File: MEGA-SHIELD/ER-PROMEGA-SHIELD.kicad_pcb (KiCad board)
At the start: 2 copper layers, 80 parts, among them J1 12V, J10 Screw_Terminal_01x10, J11 Screw_Terminal_01x07, J12 Conn_01x03_Female, J13 Screw_Terminal_01x04, J14 Conn_01x03_Female, J15 Screw_Terminal_01x04, J16 Conn_01x03_Female, J17 Screw_Terminal_01x04, J18 1x3, J19 Screw_Terminal_01x07, J2 Conn_01x03_Female, J3 Screw_Terminal_01x04, J4 Screw_Terminal_01x10, J5 Screw_Terminal_01x06, J6 Screw_Terminal_01x06, J7 Screw_Terminal_01x10, J8 Screw_Terminal_01x04, J9 Screw_Terminal_01x10, K1 G5LE-1, K2 G5LE-1, K3 G5LE-1, K4 G5LE-1, Q1 2N7002H, Q2 2N7002H, Q3 2N7002H, Q4 2N7002H, U1 PC817, U2 PC817, U3 PC817, U4 PC817

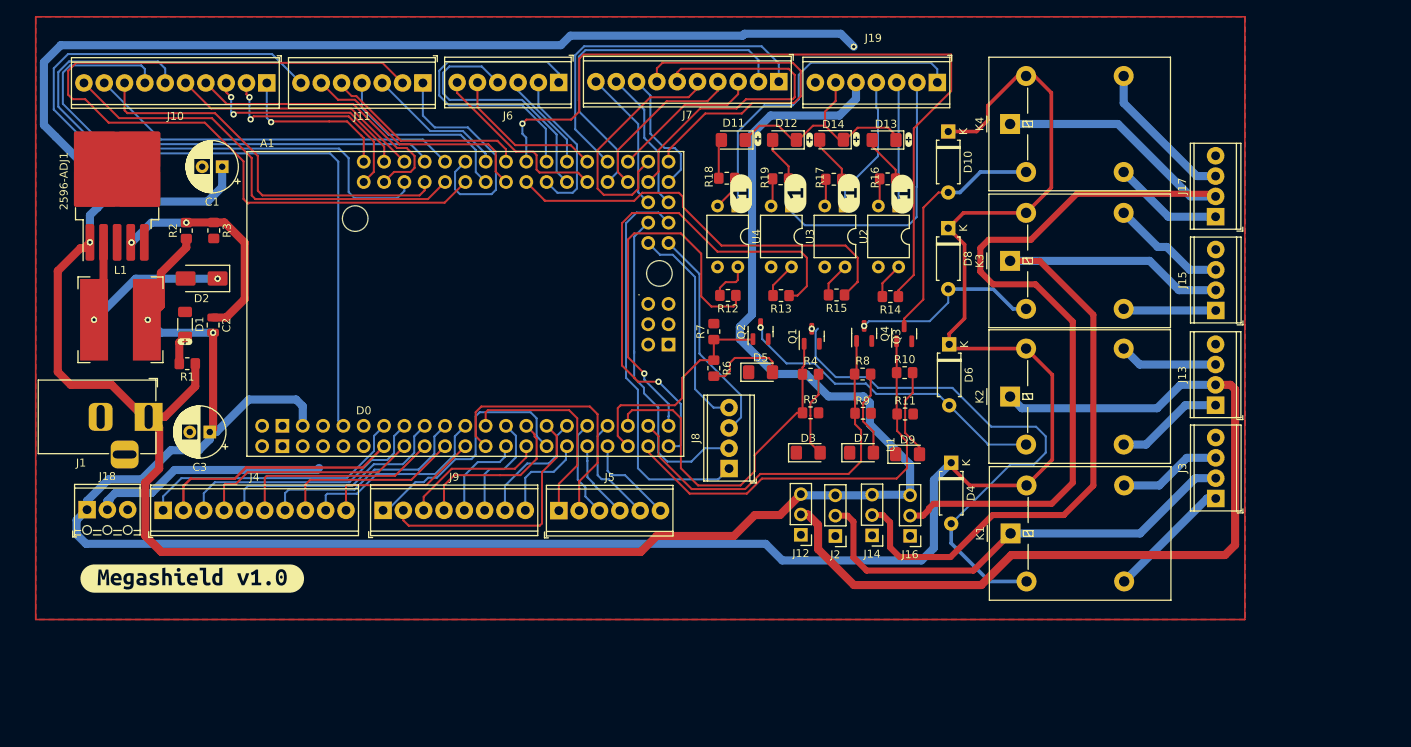
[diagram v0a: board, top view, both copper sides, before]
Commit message: develop: version 1.1
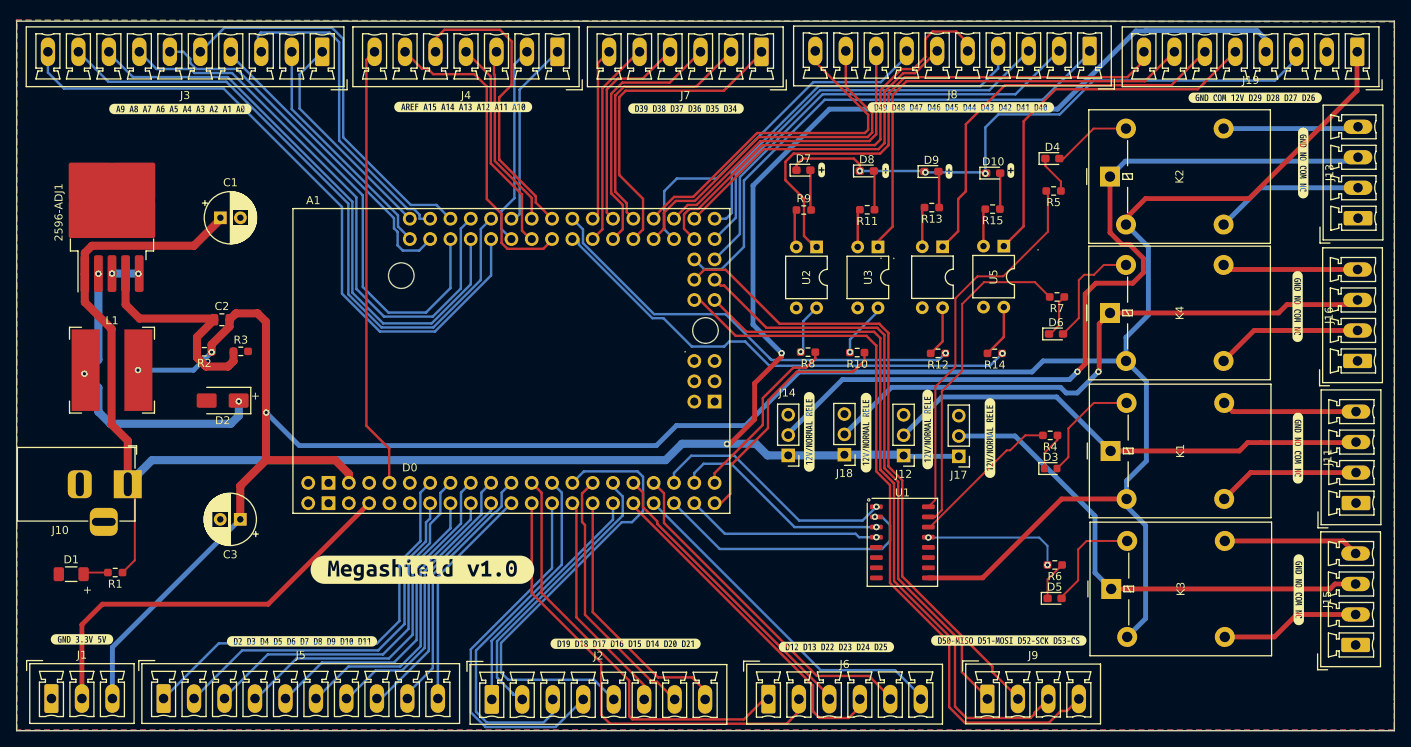
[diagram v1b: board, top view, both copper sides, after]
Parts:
- removed the D10 at (186.6, 73.1)
- removed the D7 at (175.7, 113.3)
- removed the D8 at (186.6, 85.2)
- removed the D9 at (181.5, 113.5)
- removed the J2 at (172.5, 123.7)
- removed the J3 at (220.0, 119.0)
- removed Q1, Q2, Q3, Q4: 2N7002H, Package_TO_SOT_SMD:SOT-23
- removed the R10 at (181.1, 103.3)
- removed the R11 at (181.2, 108.4)
- removed the R8 at (175.9, 103.4)
- removed the R9 at (175.9, 108.3)
- removed kibuzzard-653EC514 (x4): G***, kibuzzard-653EC514
- removed the kibuzzard-653EC60C at (91.2, 99.4)
- added J11: Screw_Terminal_01x03, Connector_Phoenix_MC:PhoenixContact_MCV_1,5_4-G-3.81_1x04_P3.81mm_Vertical, F.Cu at (237.6, 119.6)
- added J18: Conn_01x03_Female, Connector_PinHeader_2.54mm:PinHeader_1x03_P2.54mm_Vertical, F.Cu at (173.6, 113.5)
- added U1: ULN2003, PCM_Package_SO_AKL:SOP-16_4.55x10.3mm_P1.27mm, F.Cu at (180.8, 124.5)
- added kibuzzard-65BC3466: G***, kibuzzard-65BC3466, F.Cu at (90.6, 70.3)
- added kibuzzard-65BC3498: G***, kibuzzard-65BC3498, F.Cu at (126.0, 70.0)
- added kibuzzard-65BC34CA: G***, kibuzzard-65BC34CA, F.Cu at (153.8, 70.2)
- added kibuzzard-65BC34FE: G***, kibuzzard-65BC34FE, F.Cu at (188.2, 70.1)
- added kibuzzard-65BC3573: G***, kibuzzard-65BC3573, F.Cu at (224.9, 68.9)
- added kibuzzard-65BC35D6: G***, kibuzzard-65BC35D6, F.Cu at (78.3, 136.6)
- added kibuzzard-65BC363F: G***, kibuzzard-65BC363F, F.Cu at (105.8, 136.8)
- added kibuzzard-65BC3690: G***, kibuzzard-65BC3690, F.Cu at (146.2, 137.2)
- added kibuzzard-65BC36E0: G***, kibuzzard-65BC36E0, F.Cu at (172.6, 137.6)
- added kibuzzard-65BC3745: G***, kibuzzard-65BC3745, F.Cu at (194.2, 136.8)
- added kibuzzard-65BC37BD: G***, kibuzzard-65BC37BD, F.Cu at (176.3, 110.8)
- added kibuzzard-65BC37BD: G***, kibuzzard-65BC37BD, F.Cu at (169.2, 110.7)
- added kibuzzard-65BC37BD: G***, kibuzzard-65BC37BD, F.Cu at (184.0, 110.4)
- added kibuzzard-65BC37BD: G***, kibuzzard-65BC37BD, F.Cu at (191.8, 111.4)
- added kibuzzard-65BC3814: G***, kibuzzard-65BC3814, F.Cu at (230.4, 130.4)
- added kibuzzard-65BC3814: G***, kibuzzard-65BC3814, F.Cu at (230.9, 77.0)
- added kibuzzard-65BC3814: G***, kibuzzard-65BC3814, F.Cu at (230.2, 95.0)
- added kibuzzard-65BC3814: G***, kibuzzard-65BC3814, F.Cu at (230.3, 112.7)
- 2596-ADJ1: value LM2596S-5 -> REGULADOR ADJ
- D10: renamed from D14; footprint LED_SMD:LED_1206_3216Metric_Pad1.42x1.75mm_HandSolder -> LED_SMD:LED_0603_1608Metric_Pad1.05x0.95mm_HandSolder
- D3: value LEDRELE -> LED; footprint LED_SMD:LED_1206_3216Metric_Pad1.42x1.75mm_HandSolder -> LED_SMD:LED_0603_1608Metric
- D4, D6: value 1N5400 -> LED; footprint Diode_THT:D_A-405_P7.62mm_Horizontal -> LED_SMD:LED_0603_1608Metric_Pad1.05x0.95mm_HandSolder
- D5: value LEDRELE -> LED; footprint LED_SMD:LED_1206_3216Metric_Pad1.42x1.75mm_HandSolder -> LED_SMD:LED_0603_1608Metric_Pad1.05x0.95mm_HandSolder
- D7: renamed from D11; footprint LED_SMD:LED_1206_3216Metric_Pad1.42x1.75mm_HandSolder -> LED_SMD:LED_0603_1608Metric_Pad1.05x0.95mm_HandSolder
- D8: renamed from D12; footprint LED_SMD:LED_1206_3216Metric_Pad1.42x1.75mm_HandSolder -> LED_SMD:LED_0603_1608Metric_Pad1.05x0.95mm_HandSolder
- D9: renamed from D13; footprint LED_SMD:LED_1206_3216Metric_Pad1.42x1.75mm_HandSolder -> LED_SMD:LED_0603_1608Metric_Pad1.05x0.95mm_HandSolder
- J1: renamed from J18; footprint TerminalBlock_Phoenix:TerminalBlock_Phoenix_MPT-0,5-3-2.54_1x03_P2.54mm_Horizontal -> Connector_Phoenix_MC:PhoenixContact_MCV_1,5_3-G-3.81_1x03_P3.81mm_Vertical
- J13, J15: value Screw_Terminal_01x04 -> Screw_Terminal_01x03; footprint TerminalBlock_Phoenix:TerminalBlock_Phoenix_MPT-0,5-4-2.54_1x04_P2.54mm_Horizontal -> Connector_Phoenix_MC:PhoenixContact_MCV_1,5_4-G-3.81_1x04_P3.81mm_Vertical
- J16: value Conn_01x03_Female -> Screw_Terminal_01x03; footprint Connector_PinHeader_2.54mm:PinHeader_1x03_P2.54mm_Vertical -> Connector_Phoenix_MC:PhoenixContact_MCV_1,5_4-G-3.81_1x04_P3.81mm_Vertical
- J17: value Screw_Terminal_01x04 -> Conn_01x03_Female; footprint TerminalBlock_Phoenix:TerminalBlock_Phoenix_MPT-0,5-4-2.54_1x04_P2.54mm_Horizontal -> Connector_PinHeader_2.54mm:PinHeader_1x03_P2.54mm_Vertical
- J19: value Screw_Terminal_01x07 -> ENTRADAS OPTOS; footprint TerminalBlock_Phoenix:TerminalBlock_Phoenix_MPT-0,5-7-2.54_1x07_P2.54mm_Horizontal -> Connector_Phoenix_MC:PhoenixContact_MCV_1,5_8-G-3.81_1x08_P3.81mm_Vertical
- J2: renamed from J9; footprint TerminalBlock_Phoenix:TerminalBlock_Phoenix_MPT-0,5-8-2.54_1x08_P2.54mm_Horizontal -> Connector_Phoenix_MC:PhoenixContact_MCV_1,5_8-G-3.81_1x08_P3.81mm_Vertical
- J3: renamed from J10; footprint TerminalBlock_Phoenix:TerminalBlock_Phoenix_MPT-0,5-10-2.54_1x10_P2.54mm_Horizontal -> Connector_Phoenix_MC:PhoenixContact_MCV_1,5_10-G-3.81_1x10_P3.81mm_Vertical
- J4: renamed from J11; footprint TerminalBlock_Phoenix:TerminalBlock_Phoenix_MPT-0,5-7-2.54_1x07_P2.54mm_Horizontal -> Connector_Phoenix_MC:PhoenixContact_MCV_1,5_7-G-3.81_1x07_P3.81mm_Vertical
- J5: renamed from J4; footprint TerminalBlock_Phoenix:TerminalBlock_Phoenix_MPT-0,5-10-2.54_1x10_P2.54mm_Horizontal -> Connector_Phoenix_MC:PhoenixContact_MCV_1,5_10-G-3.81_1x10_P3.81mm_Vertical
- J6: renamed from J5; footprint TerminalBlock_Phoenix:TerminalBlock_Phoenix_MPT-0,5-6-2.54_1x06_P2.54mm_Horizontal -> Connector_Phoenix_MC:PhoenixContact_MCV_1,5_6-G-3.81_1x06_P3.81mm_Vertical
- J7: renamed from J6; footprint TerminalBlock_Phoenix:TerminalBlock_Phoenix_MPT-0,5-6-2.54_1x06_P2.54mm_Horizontal -> Connector_Phoenix_MC:PhoenixContact_MCV_1,5_6-G-3.81_1x06_P3.81mm_Vertical
- J8: renamed from J7; footprint TerminalBlock_Phoenix:TerminalBlock_Phoenix_MPT-0,5-10-2.54_1x10_P2.54mm_Horizontal -> Connector_Phoenix_MC:PhoenixContact_MCV_1,5_10-G-3.81_1x10_P3.81mm_Vertical
- J9: renamed from J8; footprint TerminalBlock_Phoenix:TerminalBlock_Phoenix_MPT-0,5-4-2.54_1x04_P2.54mm_Horizontal -> Connector_Phoenix_MC:PhoenixContact_MCV_1,5_4-G-3.81_1x04_P3.81mm_Vertical
- K1: value G5LE-1 -> Rele3
- K2: value G5LE-1 -> Rele1
- K3: value G5LE-1 -> Rele4
- K4: value G5LE-1 -> Rele2
- R1, R2, R3: footprint Resistor_SMD:R_0805_2012Metric_Pad1.20x1.40mm_HandSolder -> Resistor_SMD:R_0603_1608Metric_Pad0.98x0.95mm_HandSolder
- R10: renamed from R13; footprint Resistor_SMD:R_0805_2012Metric_Pad1.20x1.40mm_HandSolder -> Resistor_SMD:R_0603_1608Metric_Pad0.98x0.95mm_HandSolder
- R11: renamed from R19; footprint Resistor_SMD:R_0805_2012Metric_Pad1.20x1.40mm_HandSolder -> Resistor_SMD:R_0603_1608Metric_Pad0.98x0.95mm_HandSolder
- R12: renamed from R14; footprint Resistor_SMD:R_0805_2012Metric_Pad1.20x1.40mm_HandSolder -> Resistor_SMD:R_0603_1608Metric_Pad0.98x0.95mm_HandSolder
- R13: renamed from R16; footprint Resistor_SMD:R_0805_2012Metric_Pad1.20x1.40mm_HandSolder -> Resistor_SMD:R_0603_1608Metric_Pad0.98x0.95mm_HandSolder
- R14: renamed from R15; footprint Resistor_SMD:R_0805_2012Metric_Pad1.20x1.40mm_HandSolder -> Resistor_SMD:R_0603_1608Metric_Pad0.98x0.95mm_HandSolder
- R15: renamed from R17; footprint Resistor_SMD:R_0805_2012Metric_Pad1.20x1.40mm_HandSolder -> Resistor_SMD:R_0603_1608Metric_Pad0.98x0.95mm_HandSolder
- R4, R6: value 1k -> R; footprint Resistor_SMD:R_0805_2012Metric_Pad1.20x1.40mm_HandSolder -> Resistor_SMD:R_0603_1608Metric_Pad0.98x0.95mm_HandSolder
- R5, R7: value 10K -> R; footprint Resistor_SMD:R_0805_2012Metric_Pad1.20x1.40mm_HandSolder -> Resistor_SMD:R_0603_1608Metric_Pad0.98x0.95mm_HandSolder
- R8: renamed from R12; footprint Resistor_SMD:R_0805_2012Metric_Pad1.20x1.40mm_HandSolder -> Resistor_SMD:R_0603_1608Metric_Pad0.98x0.95mm_HandSolder
- R9: renamed from R18; footprint Resistor_SMD:R_0805_2012Metric_Pad1.20x1.40mm_HandSolder -> Resistor_SMD:R_0603_1608Metric_Pad0.98x0.95mm_HandSolder
- U2: renamed from U4; value PC817 -> OPTO1
- U3: value PC817 -> OPTO2
- U4: renamed from U1; value PC817 -> OPTO3
- U5: renamed from U2; value PC817 -> OPTO4
- moved J16 60.1 mm to (237.7, 101.8), turned to 90 degrees
- moved J19 52.6 mm to (237.7, 63.1)
- moved R6 49.2 mm to (199.9, 127.3), turned to 180 degrees
- moved D5 46.4 mm to (199.9, 131.5)
- moved J15 45.3 mm to (237.5, 137.3)
- moved J17 43.9 mm to (187.9, 113.7), turned to 180 degrees
- moved J9 43.3 mm to (191.5, 144.1), turned to 0 degrees
- moved R7 43.1 mm to (200.2, 93.8), turned to 180 degrees
- moved K3 42.9 mm to (206.9, 130.3)
- moved R5 41.1 mm to (199.8, 80.5), turned to 180 degrees
- moved D4 40.1 mm to (199.6, 76.5), turned to 0 degrees
- moved J8 39.0 mm to (204.2, 63.0)
- moved J6 35.2 mm to (164.1, 144.1)
- moved D1 34.3 mm to (77.0, 128.4), turned to 0 degrees
- moved R4 30.9 mm to (199.3, 111.1), turned to 180 degrees
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- renumbered J1 to J10
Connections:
- A1 pad 3V31: Net-(J18-Pin_2) -> unconnected-(A1-3.3V-Pad3V31)
- A1 pad 3V32: unconnected-(A1-3.3V-Pad3V32) -> Net-(J1-Pin_2)
- A1 pad D26: /sig -> /sig1
- A1 pad D27: /sig1 -> /sig2
- A1 pad D28: /sig2 -> /sig3
- A1 pad D29: /sig3 -> /sig4
- A1 pad D34: Net-(J6-Pin_1) (its old number) -> Net-(J7-Pin_6)
- A1 pad D35: Net-(J6-Pin_2) (its old number) -> Net-(J7-Pin_5)
- A1 pad D36: Net-(J6-Pin_3) (its old number) -> Net-(J7-Pin_4)
- A1 pad D37: Net-(J6-Pin_4) (its old number) -> Net-(J7-Pin_3)
- A1 pad D38: Net-(J6-Pin_5) (its old number) -> Net-(J7-Pin_2)
- A1 pad D39: Net-(J6-Pin_6) (its old number) -> Net-(J7-Pin_1)
- A1 pad D40: Net-(J7-Pin_1) -> Net-(J8-Pin_10)
- A1 pad D41: Net-(J7-Pin_2) -> Net-(J8-Pin_9)
- A1 pad D42: Net-(J7-Pin_3) -> Net-(J8-Pin_8)
- A1 pad D43: Net-(J7-Pin_4) -> Net-(J8-Pin_7)
- A1 pad D44: Net-(J7-Pin_5) -> Net-(J8-Pin_6)
- A1 pad D45: Net-(J7-Pin_6) -> Net-(J8-Pin_5)
- A1 pad D46: Net-(J7-Pin_7) -> Net-(J8-Pin_4)
- A1 pad D47: Net-(J7-Pin_8) -> Net-(J8-Pin_3)
- A1 pad D48: Net-(J7-Pin_9) -> Net-(J8-Pin_2)
- A1 pad D49: Net-(J7-Pin_10) -> Net-(J8-Pin_1)
- D3 pad 1: GND -> Net-(D3-K)
- D4 pad 1: +5V -> Net-(D4-K)
- D5 pad 1: GND -> Net-(D5-K)
- D6 pad 1: +5V -> Net-(D6-K)
- J1 pad 1: +5V -> GND
- J1 pad 2: Net-(J18-Pin_2) -> Net-(J1-Pin_2)
- J1 pad 3: GND -> +5V
- J12 pad 1: unconnected-(J12-Pin_1-Pad1) -> +12V
- J12 pad 2: Net-(J12-Pin_2) -> /uln2003/COM3
- J12 pad 3: +12V -> unconnected-(J12-Pin_3-Pad3)
- J13 pad 1: Net-(J13-Pin_1) -> GND
- J13 pad 2: Net-(J12-Pin_2) -> /uln2003/NO1
- J13 pad 3: Net-(J13-Pin_3) -> /uln2003/COM1
- J13 pad 4: GND -> /uln2003/NC1
- J14 pad 1: unconnected-(J14-Pin_1-Pad1) -> +12V
- J14 pad 2: Net-(J14-Pin_2) -> /uln2003/COM1
- J14 pad 3: +12V -> unconnected-(J14-Pin_3-Pad3)
- J15 pad 1: Net-(J15-Pin_1) -> GND
- J15 pad 2: Net-(J14-Pin_2) -> /uln2003/NO4
- J15 pad 3: Net-(J15-Pin_3) -> /uln2003/COM4
- J15 pad 4: GND -> /uln2003/NC4
- J16 pad 1: unconnected-(J16-Pin_1-Pad1) -> GND
- J16 pad 2: Net-(J16-Pin_2) -> /uln2003/NO2
- J16 pad 3: +12V -> /uln2003/COM2
- J17 pad 1: Net-(J17-Pin_1) -> +12V
- J17 pad 2: Net-(J16-Pin_2) -> /uln2003/COM4
- J17 pad 3: Net-(J17-Pin_3) -> unconnected-(J17-Pin_3-Pad3)
- J19 pad 1: /optos/SIG1 -> +5V
- J19 pad 2: /optos/SIG2 -> GND
- J19 pad 3: /optos/SIG3 -> /optos/COM
- J19 pad 4: /optos/SIG4 -> +12V
- J19 pad 5: +12V -> /optos/SIG4
- J19 pad 6: /optos/COM -> /optos/SIG3
- J19 pad 7: GND -> /optos/SIG2
- J2 pad 1: Net-(A1-D19/RX1) -> Net-(A1-D21/SCL)
- J2 pad 2: Net-(A1-D18/TX1) -> Net-(A1-D20/SDA)
- J2 pad 3: Net-(A1-D17/RX2) -> Net-(A1-D14/TX3)
- J2 pad 4: Net-(A1-D16/TX2) -> Net-(A1-D15/RX3)
- J2 pad 5: Net-(A1-D15/RX3) -> Net-(A1-D16/TX2)
- J2 pad 6: Net-(A1-D14/TX3) -> Net-(A1-D17/RX2)
- J2 pad 7: Net-(A1-D20/SDA) -> Net-(A1-D18/TX1)
- J2 pad 8: Net-(A1-D21/SCL) -> Net-(A1-D19/RX1)
- J7 pad 1: Net-(J6-Pin_1) (its old number) -> Net-(J7-Pin_1)
- J7 pad 2: Net-(J6-Pin_2) (its old number) -> Net-(J7-Pin_2)
- J7 pad 3: Net-(J6-Pin_3) (its old number) -> Net-(J7-Pin_3)
- J7 pad 4: Net-(J6-Pin_4) (its old number) -> Net-(J7-Pin_4)
- J7 pad 5: Net-(J6-Pin_5) (its old number) -> Net-(J7-Pin_5)
- J7 pad 6: Net-(J6-Pin_6) (its old number) -> Net-(J7-Pin_6)
- J8 pad 1: Net-(J7-Pin_1) -> Net-(J8-Pin_1)
- J8 pad 10: Net-(J7-Pin_10) -> Net-(J8-Pin_10)
- J8 pad 2: Net-(J7-Pin_2) -> Net-(J8-Pin_2)
- J8 pad 3: Net-(J7-Pin_3) -> Net-(J8-Pin_3)
- J8 pad 4: Net-(J7-Pin_4) -> Net-(J8-Pin_4)
- J8 pad 5: Net-(J7-Pin_5) -> Net-(J8-Pin_5)
- J8 pad 6: Net-(J7-Pin_6) -> Net-(J8-Pin_6)
- J8 pad 7: Net-(J7-Pin_7) -> Net-(J8-Pin_7)
- J8 pad 8: Net-(J7-Pin_8) -> Net-(J8-Pin_8)
- J8 pad 9: Net-(J7-Pin_9) -> Net-(J8-Pin_9)
- K1 pad 1: Net-(J2-Pin_2) -> /uln2003/COM3
- K1 pad 2: Net-(D4-A) -> +5V
- K1 pad 3: Net-(J3-Pin_1) (its old number) -> /uln2003/NO3
- K1 pad 4: Net-(J3-Pin_3) (its old number) -> /uln2003/NC3
- K1 pad 5: +5V -> Net-(D3-A)
- K2 pad 1: Net-(J12-Pin_2) -> /uln2003/COM1
- K2 pad 2: Net-(D6-A) -> +5V
- K2 pad 3: Net-(J13-Pin_1) -> /uln2003/NO1
- K2 pad 4: Net-(J13-Pin_3) -> /uln2003/NC1
- K2 pad 5: +5V -> Net-(D4-A)
- K3 pad 1: Net-(J14-Pin_2) -> /uln2003/COM4
- K3 pad 2: Net-(D8-A) (its old number) -> +5V
- K3 pad 3: Net-(J15-Pin_1) -> /uln2003/NO4
- K3 pad 4: Net-(J15-Pin_3) -> /uln2003/NC4
- K3 pad 5: +5V -> Net-(D5-A)
- K4 pad 1: Net-(J16-Pin_2) -> /uln2003/COM2
- K4 pad 2: Net-(D10-A) (its old number) -> +5V
- K4 pad 3: Net-(J17-Pin_1) -> /uln2003/NO2
- K4 pad 4: Net-(J17-Pin_3) -> /uln2003/NC2
- K4 pad 5: +5V -> Net-(D6-A)
- R4 pad 1: /sig -> Net-(D3-K)
- R4 pad 2: Net-(D3-A) -> /uln2003/RELE3
- R5 pad 1: /sig -> Net-(D4-K)
- R5 pad 2: GND -> /uln2003/RELE1
- R6 pad 1: /sig1 -> Net-(D5-K)
- R6 pad 2: Net-(D5-A) -> /uln2003/RELE4
- R7 pad 1: /sig1 -> Net-(D6-K)
- R7 pad 2: GND -> /uln2003/RELE2
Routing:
- net Net-(J16-Pin_2): track 121.2 -> 0.00 mm
- net Net-(J12-Pin_2): track 111.4 -> 0.00 mm
- net /uln2003/COM1: track 0.00 -> 104.3 mm, vias 0 -> 1
- net +12V: track 382.3 -> 279.7 mm
- net Net-(J14-Pin_2): track 97.2 -> 0.00 mm
- net Net-(J4-Pin_2): track 105.4 -> 25.3 mm
- net /uln2003/COM2: track 0.00 -> 75.1 mm, vias 0 -> 1
- net Net-(J8-Pin_1): track 0.00 -> 66.2 mm
- net Net-(A1-D53_CS): track 26.8 -> 92.3 mm
- net /uln2003/COM4: track 0.00 -> 61.9 mm
- net /uln2003/COM3: track 0.00 -> 61.8 mm
- net Net-(A1-D52_SCK): track 27.6 -> 85.9 mm
- net Net-(D4-A): track 67.9 -> 9.88 mm, vias 1 -> 0
- net Net-(J8-Pin_2): track 0.00 -> 57.8 mm
- net Net-(J2-Pin_2): track 57.8 -> 0.00 mm
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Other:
- board outline added: 172.2 x 88.7 mm
- board text added: "+"
- board text added: "."
